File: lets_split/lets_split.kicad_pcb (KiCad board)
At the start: 2 copper layers, 114.2 x 82 mm, 66 parts, among them J1 Speaker, P1 USB-rewire, P2 USB_OTG, P3 WS2812, P3 WS2812-Strip, P4 Conn_01x04, P5 USB_OTG, P6 Conn_01x04, SW1 SW_PUSH, SW10 SW_PUSH, SW11 SW_PUSH, SW12 SW_PUSH, SW13 SW_PUSH, SW14 SW_PUSH, SW15 SW_PUSH, SW16 SW_PUSH, SW17 SW_PUSH, SW18 SW_PUSH, SW19 SW_PUSH, SW2 SW_PUSH, SW20 SW_PUSH, SW21 SW_PUSH, SW22 SW_PUSH, SW23 SW_PUSH, SW24 SW_PUSH, SW3 SW_PUSH, SW4 SW_PUSH, SW5 SW_PUSH, SW6 SW_PUSH, SW7 SW_PUSH, SW8 SW_PUSH, SW9 SW_PUSH, U1 ArduinoProMicro

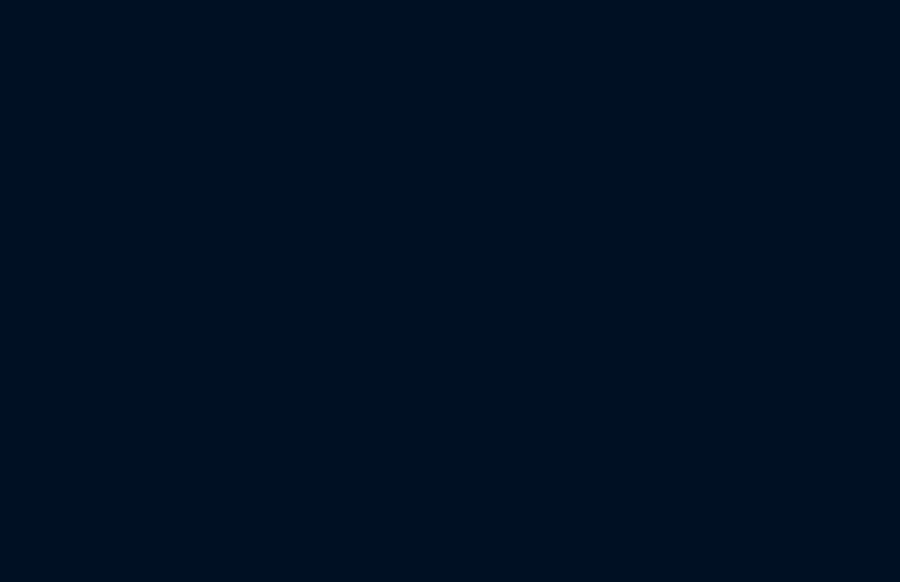
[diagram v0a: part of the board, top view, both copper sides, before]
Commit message: First commit for mcu version
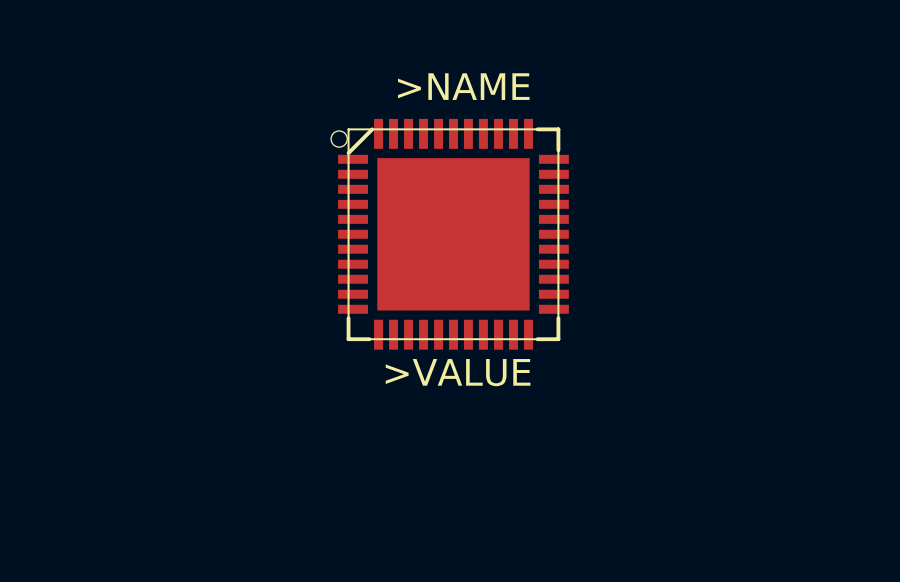
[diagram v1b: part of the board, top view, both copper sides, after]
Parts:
- added >NAME: >VALUE, SeeedOPL-IC-2016:QFN44G-0.5-7X7MM, F.Cu at (149.7, 45.3)
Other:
- net class Default: trace_width 0.1524 -> 0.25
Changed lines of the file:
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@@
     (tracks 845)
     (zones 0)
-    (modules 66)
+    (modules 67)
     (nets 54)
   )
@@
   )
   (setup
-    (last_trace_width 0.1524)
+    (last_trace_width 0.25)
     (user_trace_width 0.2032)
     (user_trace_width 0.4064)
@@
   (net_class Default "This is the default net class."
     (clearance 0.2032)
-    (trace_width 0.1524)
+    (trace_width 0.25)
     (via_dia 0.8)
     (via_drill 0.4)
@@
     (add_net row3)
   )
+  (module SeeedOPL-IC-2016:QFN44G-0.5-7X7MM (layer F.Cu)
+    (at 149.733 45.339)
+    (attr smd)
+    (fp_text reference >NAME (at 0.3175 -4.8895) (layer F.SilkS)
+      (effects (font (size 0.889 0.889) (thickness 0.1016)))
+    )
+    (fp_text value >VALUE (at 0.127 4.6355) (layer F.SilkS)
+      (effects (font (size 0.889 0.889) (thickness 0.1016)))
+    )
+    (fp_circle (center -3.81 -3.175) (end -4.0005 -3.3655) (layer F.SilkS) (width 0))
+    (fp_line (start 3.49758 -3.49758) (end 2.79908 -3.49758) (layer F.SilkS) (width 0.127))
+    (fp_line (start 3.49758 -2.79908) (end 3.49758 -3.49758) (layer F.SilkS) (width 0.127))
+    (fp_line (start 3.49758 3.49758) (end 3.49758 2.79908) (layer F.SilkS) (width 0.127))
+    (fp_line (start 2.79908 3.49758) (end 3.49758 3.49758) (layer F.SilkS) (width 0.127))
+    (fp_line (start -3.49758 3.49758) (end -2.79908 3.49758) (layer F.SilkS) (width 0.127))
+    (fp_line (start -3.49758 2.79908) (end -3.49758 3.49758) (layer F.SilkS) (width 0.127))
+    (fp_line (start -3.49758 -2.70764) (end -2.70764 -3.49758) (layer F.SilkS) (width 0.127))
+    (fp_line (start -3.49758 3.49758) (end -3.49758 -3.49758) (layer F.SilkS) (width 0.06604))
+    (fp_line (start -3.49758 -3.49758) (end 3.49758 -3.49758) (layer F.SilkS) (width 0.06604))
+    (fp_line (start 3.49758 3.49758) (end 3.49758 -3.49758) (layer F.SilkS) (width 0.06604))
+    (fp_line (start -3.49758 3.49758) (end 3.49758 3.49758) (layer F.SilkS) (width 0.06604))
+    (pad TAB smd rect (at 0 0) (size 5.08 5.08) (layers F.Cu F.Paste F.Mask))
+    (pad 44 smd rect (at -2.49936 -3.34772 90) (size 0.99822 0.29972) (layers F.Cu F.Paste F.Mask))
+    (pad 43 smd rect (at -1.99898 -3.34772 90) (size 0.99822 0.29972) (layers F.Cu F.Paste F.Mask))
+    (pad 42 smd rect (at -1.4986 -3.34772 90) (size 0.99822 0.29972) (layers F.Cu F.Paste F.Mask))
+    (pad 41 smd rect (at -0.99822 -3.34772 90) (size 0.99822 0.29972) (layers F.Cu F.Paste F.Mask))
+    (pad 40 smd rect (at -0.49784 -3.34772 90) (size 0.99822 0.29972) (layers F.Cu F.Paste F.Mask))
+    (pad 39 smd rect (at 0 -3.34772 90) (size 0.99822 0.29972) (layers F.Cu F.Paste F.Mask))
+    (pad 38 smd rect (at 0.49784 -3.34772 90) (size 0.99822 0.29972) (layers F.Cu F.Paste F.Mask))
+    (pad 37 smd rect (at 0.99822 -3.34772 90) (size 0.99822 0.29972) (layers F.Cu F.Paste F.Mask))
+    (pad 36 smd rect (at 1.4986 -3.34772 90) (size 0.99822 0.29972) (layers F.Cu F.Paste F.Mask))
+    (pad 35 smd rect (at 1.99898 -3.34772 90) (size 0.99822 0.29972) (layers F.Cu F.Paste F.Mask))
+    (pad 34 smd rect (at 2.49936 -3.34772 90) (size 0.99822 0.29972) (layers F.Cu F.Paste F.Mask))
+    (pad 33 smd rect (at 3.34772 -2.49936) (size 0.99822 0.29972) (layers F.Cu F.Paste F.Mask))
+    (pad 32 smd rect (at 3.34772 -1.99898) (size 0.99822 0.29972) (layers F.Cu F.Paste F.Mask))
+    (pad 31 smd rect (at 3.34772 -1.4986) (size 0.99822 0.29972) (layers F.Cu F.Paste F.Mask))
+    (pad 30 smd rect (at 3.34772 -0.99822) (size 0.99822 0.29972) (layers F.Cu F.Paste F.Mask))
+    (pad 29 smd rect (at 3.34772 -0.49784) (size 0.99822 0.29972) (layers F.Cu F.Paste F.Mask))
+    (pad 28 smd rect (at 3.34772 0) (size 0.99822 0.29972) (layers F.Cu F.Paste F.Mask))
+    (pad 27 smd rect (at 3.34772 0.49784) (size 0.99822 0.29972) (layers F.Cu F.Paste F.Mask))
+    (pad 26 smd rect (at 3.34772 0.99822) (size 0.99822 0.29972) (layers F.Cu F.Paste F.Mask))
+    (pad 25 smd rect (at 3.34772 1.4986) (size 0.99822 0.29972) (layers F.Cu F.Paste F.Mask))
+    (pad 24 smd rect (at 3.34772 1.99898) (size 0.99822 0.29972) (layers F.Cu F.Paste F.Mask))
+    (pad 23 smd rect (at 3.34772 2.49936) (size 0.99822 0.29972) (layers F.Cu F.Paste F.Mask))
+    (pad 22 smd rect (at 2.49936 3.34772 270) (size 0.99822 0.29972) (layers F.Cu F.Paste F.Mask))
+    (pad 21 smd rect (at 1.99898 3.34772 270) (size 0.99822 0.29972) (layers F.Cu F.Paste F.Mask))
+    (pad 20 smd rect (at 1.4986 3.34772 270) (size 0.99822 0.29972) (layers F.Cu F.Paste F.Mask))
+    (pad 19 smd rect (at 0.99822 3.34772 270) (size 0.99822 0.29972) (layers F.Cu F.Paste F.Mask))
+    (pad 18 smd rect (at 0.49784 3.34772 270) (size 0.99822 0.29972) (layers F.Cu F.Paste F.Mask))
+    (pad 17 smd rect (at 0 3.34772 270) (size 0.99822 0.29972) (layers F.Cu F.Paste F.Mask))
+    (pad 16 smd rect (at -0.49784 3.34772 270) (size 0.99822 0.29972) (layers F.Cu F.Paste F.Mask))
+    (pad 15 smd rect (at -0.99822 3.34772 270) (size 0.99822 0.29972) (layers F.Cu F.Paste F.Mask))
+    (pad 14 smd rect (at -1.4986 3.34772 270) (size 0.99822 0.29972) (layers F.Cu F.Paste F.Mask))
+    (pad 13 smd rect (at -1.99898 3.34772 270) (size 0.99822 0.29972) (layers F.Cu F.Paste F.Mask))
+    (pad 12 smd rect (at -2.49936 3.34772 270) (size 0.99822 0.29972) (layers F.Cu F.Paste F.Mask))
+    (pad 11 smd rect (at -3.34772 2.49936 180) (size 0.99822 0.29972) (layers F.Cu F.Paste F.Mask))
+    (pad 10 smd rect (at -3.34772 1.99898 180) (size 0.99822 0.29972) (layers F.Cu F.Paste F.Mask))
+    (pad 9 smd rect (at -3.34772 1.4986 180) (size 0.99822 0.29972) (layers F.Cu F.Paste F.Mask))
+    (pad 8 smd rect (at -3.34772 0.99822 180) (size 0.99822 0.29972) (layers F.Cu F.Paste F.Mask))
+    (pad 7 smd rect (at -3.34772 0.49784 180) (size 0.99822 0.29972) (layers F.Cu F.Paste F.Mask))
+    (pad 6 smd rect (at -3.34772 0 180) (size 0.99822 0.29972) (layers F.Cu F.Paste F.Mask))
+    (pad 5 smd rect (at -3.34772 -0.49784 180) (size 0.99822 0.29972) (layers F.Cu F.Paste F.Mask))
+    (pad 4 smd rect (at -3.34772 -0.99822 180) (size 0.99822 0.29972) (layers F.Cu F.Paste F.Mask))
+    (pad 3 smd rect (at -3.34772 -1.4986 180) (size 0.99822 0.29972) (layers F.Cu F.Paste F.Mask))
+    (pad 2 smd rect (at -3.34772 -1.99898 180) (size 0.99822 0.29972) (layers F.Cu F.Paste F.Mask))
+    (pad 1 smd rect (at -3.34772 -2.49936 180) (size 0.99822 0.29972) (layers F.Cu F.Paste F.Mask))
+  )
   (module CherryMX:Kailh-socket-mirrorable (layer F.Cu)

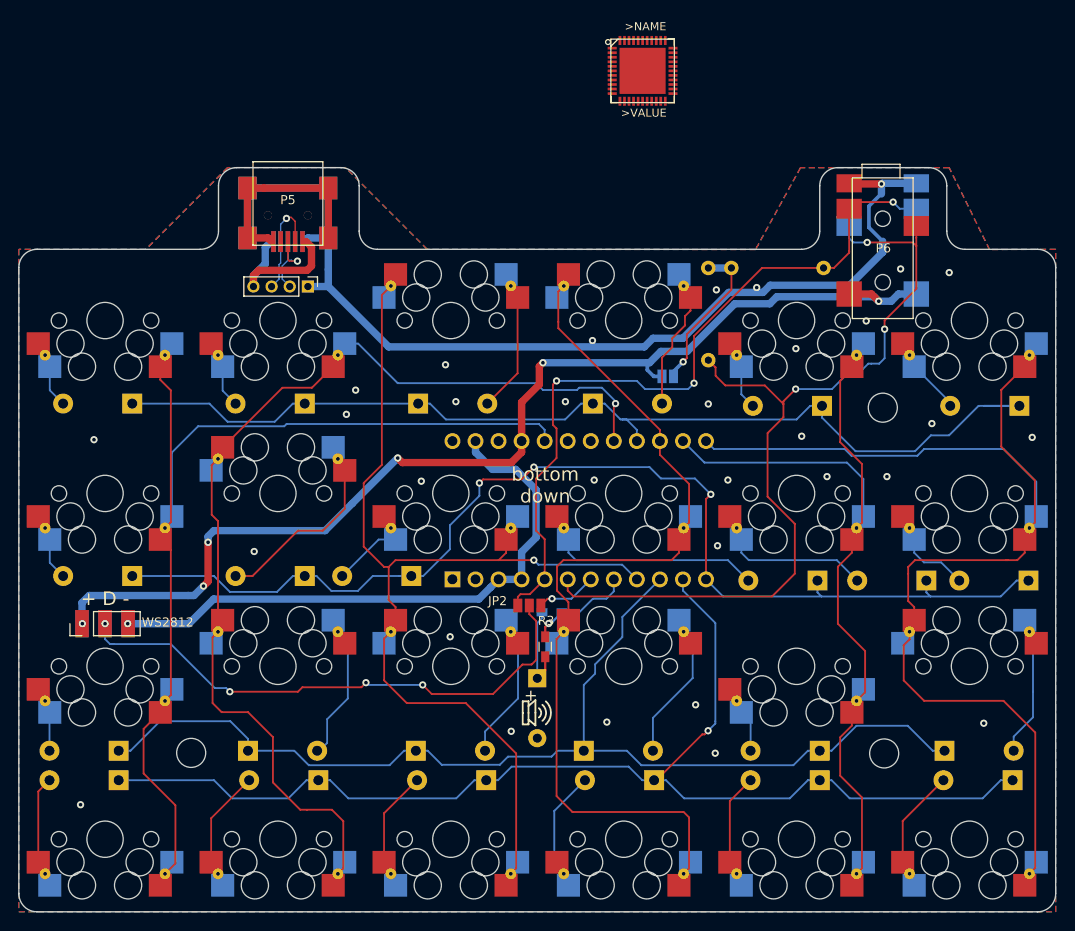
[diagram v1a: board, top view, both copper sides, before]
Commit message: Vitamins included "done"
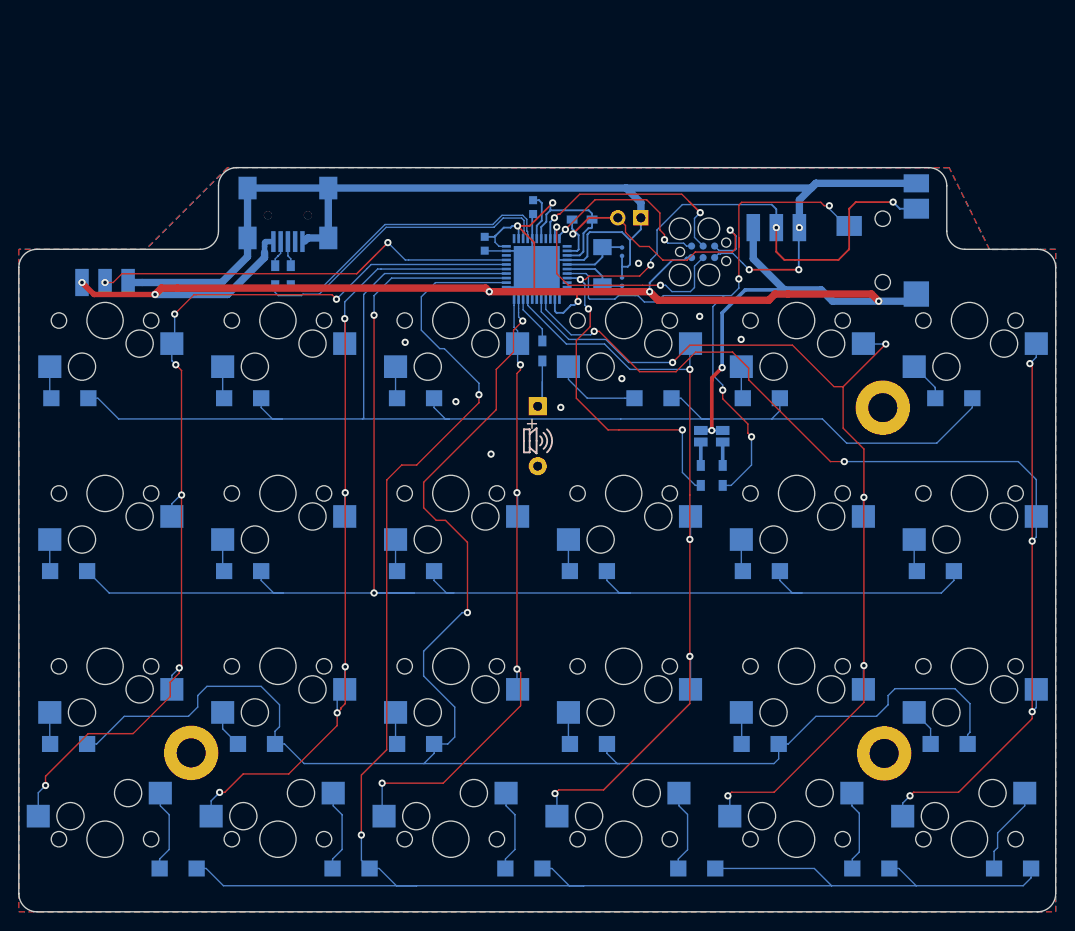
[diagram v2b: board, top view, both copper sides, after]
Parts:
- removed >NAME: >VALUE, SeeedOPL-IC-2016:QFN44G-0.5-7X7MM
- removed the P3 at (88.0, 106.2)
- removed P5: USB_OTG, Connectors:USB-Mini-B-SMD
- removed P6: Conn_01x04, Connectors:SJ-4351X-SMT
- removed the R3 at (139.0, 108.8)
- added C1: 1uF, SeeedOPL-Capacitor-2016:C0603, B.Cu at (132.3, 64.4)
- added C2: 8pF, SeeedOPL-Capacitor-2016:C0402, B.Cu at (147.5, 68.6)
- added C3: 8pF, SeeedOPL-Capacitor-2016:C0402, B.Cu at (147.5, 65.3)
- added C4: 1uF, SeeedOPL-Capacitor-2016:C0603, B.Cu at (137.7, 60.4)
- added J2: RST, Pin_Headers:Pin_Header_Straight_1x02_Pitch2.54mm, B.Cu at (149.5, 61.5)
- added J3: ISP, Jlink:J-link-needle-6pin, B.Cu at (153.9, 65.3)
- added R4: 22R, Resistors_SMD:R_0603_HandSoldering, B.Cu at (109.2, 67.9)
- added R5: 22R, Resistors_SMD:R_0603_HandSoldering, B.Cu at (111.0, 67.9)
- added R6: 4k7, Resistors_SMD:R_0603_HandSoldering, B.Cu at (143.1, 61.7)
- added Y1: Crystal, SeeedOPL-Crystal Oscillator-2016:X2-SMD-5.0X3.2X1.3MM, B.Cu at (145.3, 66.9)
- D1, D10, D11, D12, D13, D14, D15, D16, D17, D18, D19, D2, D20, D21, D22, D23, D24, D3, D4, D5, D6, D7, D8, D9: footprint Diodes_ThroughHole:D_DO-41_SOD81_P7.62mm_Horizontal -> SeeedOPL-Diode-2016:DO-214AC
- JP1: value I2C / Serial -> I2C pullup
- JP2: value DIN-selector -> I2C pullup; footprint Jumpers:Solder-jumper-12NC-23NO -> Jumpers:Solder-jumper-NO; moved to B.Cu
- P1: value USB-rewire -> WS2812>; footprint Pin_Headers:Pin_Header_Straight_1x04_Pitch2.00mm -> Wirepads:SMD_PAD_1x03_Pitch2.54mm; moved to B.Cu
- P3: value WS2812-Strip -> >WS2812
- R1, R2: footprint Resistors_ThroughHole:R_Axial_DIN0207_L6.3mm_D2.5mm_P10.16mm_Horizontal -> Resistors_SMD:R_0603_HandSoldering
- SW1, SW10, SW11, SW12, SW13, SW14, SW15, SW16, SW17, SW18, SW19, SW2, SW20, SW21, SW22, SW23, SW24, SW4, SW5, SW6, SW7, SW8, SW9: footprint CherryMX:Kailh-socket-mirrorable -> CherryMX:Kailh-socket
- SW3: footprint CherryMX:Kailh-socket-mirrorable -> Kailh-socket
- U1: value ArduinoProMicro -> ATMega32U4; footprint plug-in-modules:ArduinoProMicro -> SeeedOPL-IC-2016:QFN44G-0.5-7X7MM; moved to B.Cu
- moved P1 49.5 mm to (161.9, 62.6)
- moved P3 37.6 mm to (88.0, 68.7)
- moved J1 30.0 mm to (138.2, 82.3)
- moved R3 28.8 mm to (138.7, 76.2), turned to 270 degrees
- moved JP2 27.8 mm to (158.6, 85.6), turned to 270 degrees
- moved U1 27.0 mm to (138.1, 67.2), turned to 270 degrees
- moved D14 25.3 mm to (143.8, 100.5), turned to 0 degrees
- moved R1 23.1 mm to (156.1, 89.9), turned to 270 degrees
- moved R2 22.9 mm to (158.6, 89.9)
- moved D18 18.2 mm to (162.8, 100.5), turned to 0 degrees
- moved D4 11.7 mm to (98.6, 133.2), turned to 0 degrees
- moved D20 11.2 mm to (174.9, 133.2), turned to 0 degrees
- moved D16 10.8 mm to (155.7, 133.2), turned to 0 degrees
- moved D12 10.6 mm to (136.7, 133.2), turned to 0 degrees
- moved D8 10.4 mm to (117.6, 133.2), turned to 0 degrees
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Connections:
- JP1 pad 1: VCC -> VBUS
- JP2 pad 1: Net-(JP2-Pad1) -> VBUS
- P1 pad 1: GND -> VBUS
- P1 pad 2: /D+ -> SDA
- P1 pad 3: /D- -> GND
- P2 pad 1: Net-(P1-Pad4) -> VBUS
- P2 pad 2: /D- -> Net-(P2-Pad2)
- P2 pad 3: /D+ -> Net-(P2-Pad3)
- P3 pad 1: VCC -> VBUS
- P3 pad 2: Net-(JP2-Pad2) -> WD2812-in
- P4 pad 2: VCC -> VBUS
- R2 pad 1: Net-(JP1-Pad2) -> Net-(JP2-Pad2)
- R3 pad 1: Net-(R3-Pad1) -> buzz
- U1 pad 10: row2 -> MOSI
- U1 pad 11: row3 -> MISO
- U1 pad 12: row1 -> Net-(U1-Pad12)
- U1 pad 13: col5 -> ~RESET
- U1 pad 14: col4 -> VBUS
- U1 pad 15: col3 -> GND
- U1 pad 16: row0 -> Net-(C3-Pad1)
- U1 pad 17: col1 -> Net-(C2-Pad1)
- U1 pad 18: Net-(U1-Pad18) -> SCL/D3
- U1 pad 19: Net-(U1-Pad19) -> SDA
- U1 pad 2: Net-(U1-Pad2) -> VBUS
- U1 pad 20: col0 -> Net-(U1-Pad20)
- U1 pad 21: VCC -> Net-(U1-Pad21)
- U1 pad 24: Net-(U1-Pad24) -> VBUS
- U1 pad 3: GND -> /D-
- U1 pad 4: GND -> /D+
- U1 pad 5: SDA -> GND
- U1 pad 6: SCL/D3 -> Net-(C4-Pad1)
- U1 pad 7: Net-(JP2-Pad1) -> VBUS
- U1 pad 8: Net-(R3-Pad1) -> Net-(U1-Pad8)
- U1 pad 9: col2 -> SCK
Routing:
- net VBUS: track 0.00 -> 216.0 mm, vias 0 -> 10
- net VCC: track 123.5 -> 0.00 mm, vias 6 -> 0
- net row3: track 133.3 -> 205.5 mm, vias 1 -> 2
- net row2: track 124.3 -> 185.0 mm, vias 0 -> 2
- net Net-(JP2-Pad2): track 60.7 -> 2.58 mm, vias 4 -> 0
- net WD2812-in: track 0.00 -> 49.7 mm, vias 0 -> 2
- net col2: track 120.3 -> 72.8 mm, vias 1 -> 4
- net row1: track 125.6 -> 166.6 mm, vias 3 -> 2
- net ~RESET: track 0.00 -> 34.1 mm, vias 0 -> 2
- net row0: track 114.3 -> 147.4 mm
- net GND: track 203.1 -> 172.7 mm, vias 32 -> 11
- net SCK: track 0.00 -> 26.5 mm, vias 0 -> 2
- net MOSI: track 0.00 -> 26.4 mm, vias 0 -> 2
- net SCL/D3: track 97.6 -> 71.3 mm, vias 3 -> 4
- net col1: track 121.8 -> 96.2 mm, vias 1 -> 5
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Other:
- outline, holes or cut-outs redrawn
- net class Default: clearance 0.2032 -> 0.1524; trace_width 0.25 -> 0.1524
- rule trace_clearance: 0.2032 -> 0.1524
- board text added: "Let's Split, vitamins included"
- board text added: "Original by Wootpatoot"
- board text added: "RST"
- board text added: "by Duckle29"
- board text removed: "+ D -"
- board text removed: "- D ~D~ +"
- board text removed: "By Wootpatoot Socket Version by Duckle29"
- board text removed: "bottom down"
- board text removed: "bottom up"
